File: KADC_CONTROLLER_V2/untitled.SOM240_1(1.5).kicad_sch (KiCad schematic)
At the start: 24 parts, among them J10 ADM6-60-01.5-L-4-2-A-TR, J7 1766453, SW2 SW_MEC_5G

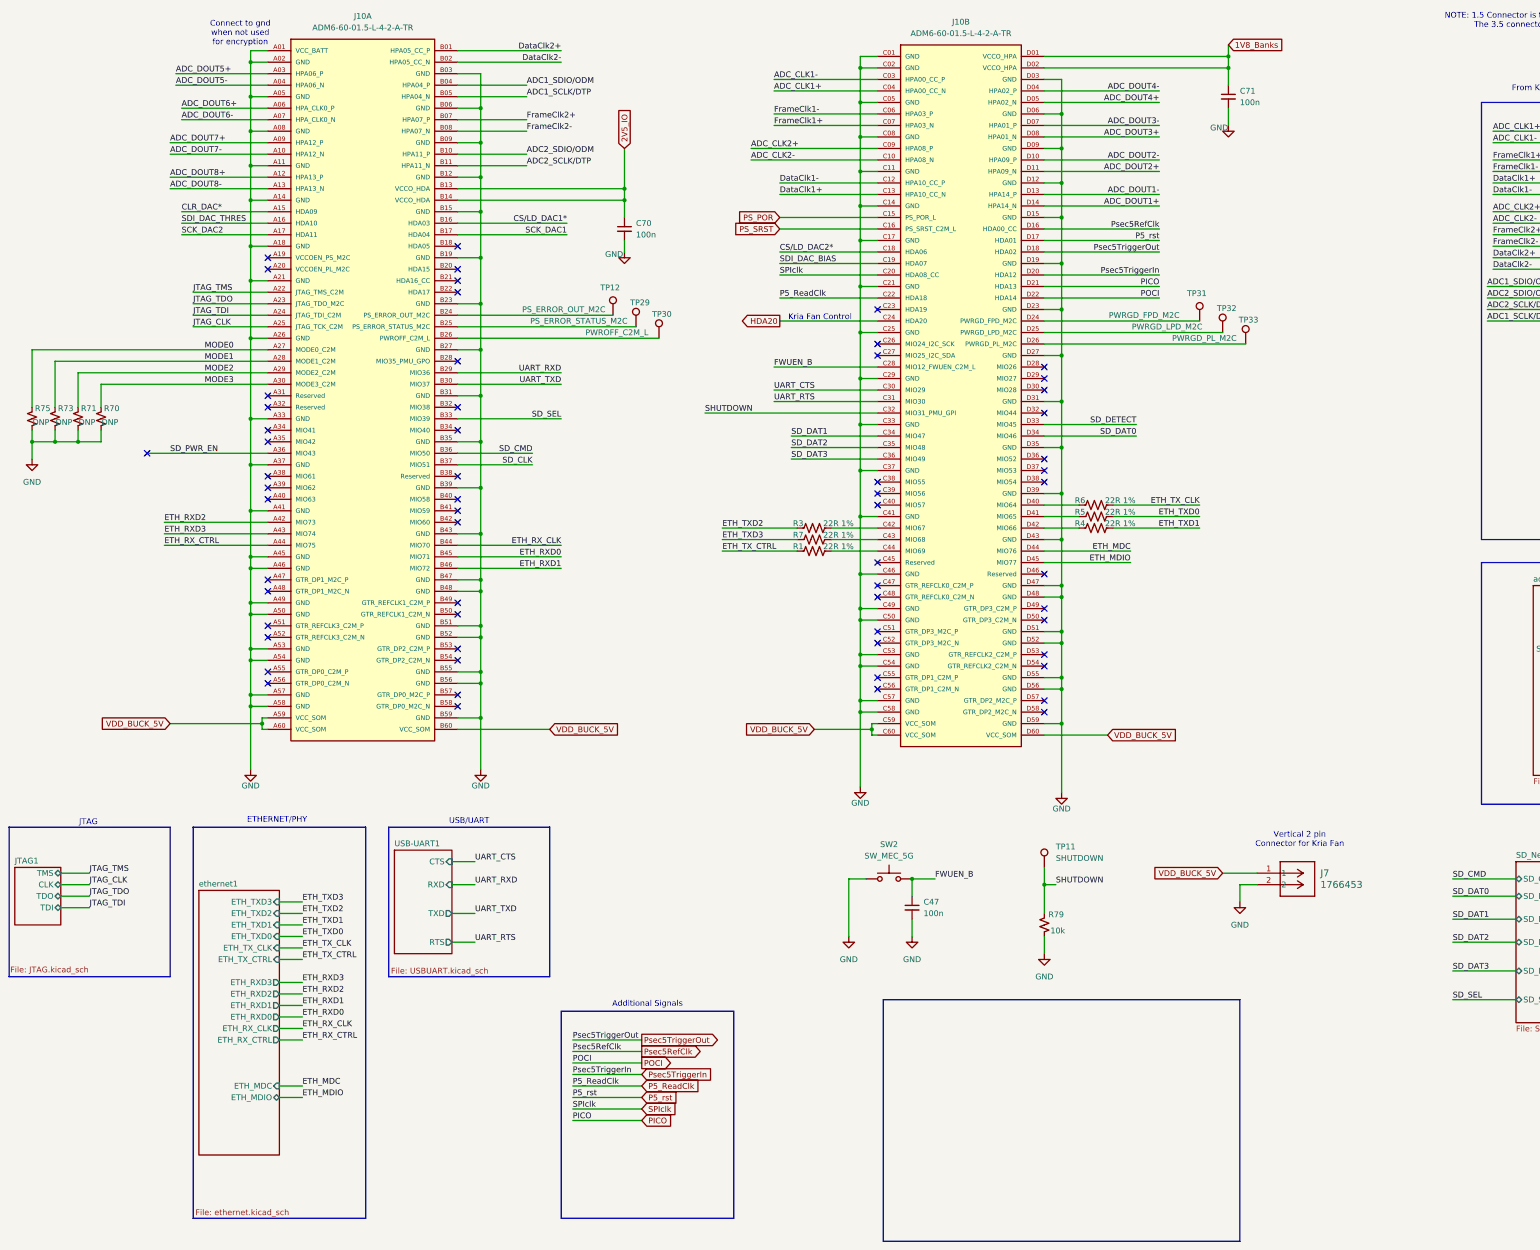
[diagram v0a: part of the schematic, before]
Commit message: many updates
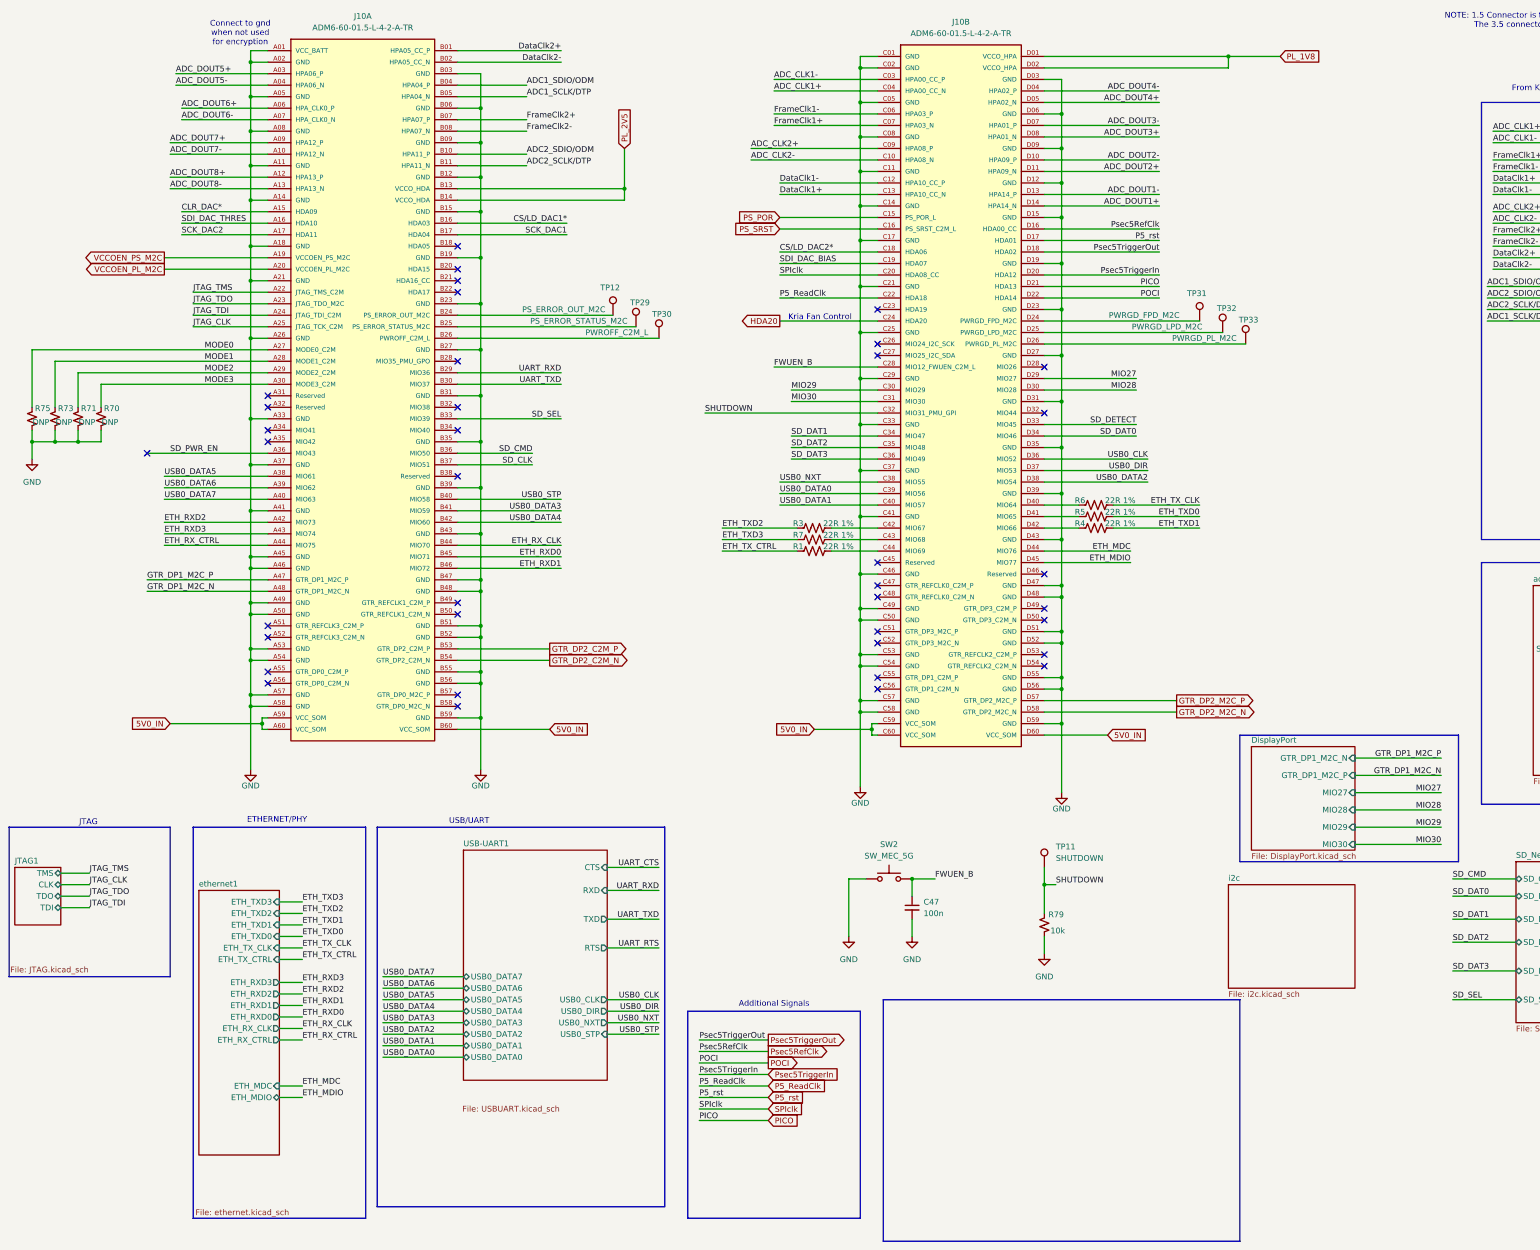
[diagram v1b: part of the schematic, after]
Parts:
- removed C70, C71: 100n, Capacitor_SMD:C_0603_1608Metric, symbol Device:C_Small
- removed J7: 1766453, 1766453:CONN_1766453, symbol PSEC5_ctrlbd:1766453
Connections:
- net UART_CTS: no longer J10.C30 (MIO29)
- net UART_RTS: no longer J10.C31 (MIO30)
- net VCCOEN_PS_M2C: now reaches J10.A19 (VCCOEN_PS_M2C)
- net VCCOEN_PL_M2C: now reaches J10.A20 (VCCOEN_PL_M2C)
- net USB0_DATA5: now reaches J10.A38 (MIO61)
- net USB0_DATA6: now reaches J10.A39 (MIO62)
- net USB0_DATA7: now reaches J10.A40 (MIO63)
- net GTR_DP1_M2C_P: now reaches J10.A47 (GTR_DP1_M2C_P)
- net GTR_DP1_M2C_N: now reaches J10.A48 (GTR_DP1_M2C_N)
- net USB0_STP: now reaches J10.B40 (MIO58)
- net USB0_DATA3: now reaches J10.B41 (MIO59)
- net USB0_DATA4: now reaches J10.B42 (MIO60)
- net GTR_DP2_C2M_P: now reaches J10.B53 (GTR_DP2_C2M_P)
- net GTR_DP2_C2M_N: now reaches J10.B54 (GTR_DP2_C2M_N)
- net USB0_NXT: now reaches J10.C38 (MIO55)
- net USB0_DATA0: now reaches J10.C39 (MIO56)
- net USB0_DATA1: now reaches J10.C40 (MIO57)
- net MIO27: now reaches J10.D29 (MIO27)
- net MIO28: now reaches J10.D30 (MIO28)
- net USB0_CLK: now reaches J10.D36 (MIO52)
- net USB0_DIR: now reaches J10.D37 (MIO53)
- net USB0_DATA2: now reaches J10.D38 (MIO54)
- net GTR_DP2_M2C_P: now reaches J10.D57 (GTR_DP2_M2C_P)
- net GTR_DP2_M2C_N: now reaches J10.D58 (GTR_DP2_M2C_N)
- net 1V8_Banks renamed PL_1V8
- net 2V5_IO renamed PL_2V5
- net VDD_BUCK_5V renamed 5V0_IN
- new net MIO29: J10.C30 (MIO29)
- new net MIO30: J10.C31 (MIO30)
- no-connect marks 60 -> 38
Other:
- added sheet DisplayPort (DisplayPort.kicad_sch)
- added sheet i2c (i2c.kicad_sch)
- sheet USB-UART1 ports: added USB0_CLK, USB0_DATA0, USB0_DATA1, USB0_DATA2, USB0_DATA3, USB0_DATA4, USB0_DATA5, USB0_DATA6, USB0_DATA7, USB0_DIR, USB0_NXT, USB0_STP; removed none
- note removed: "Vertical 2 pin Connector for Kria Fan"

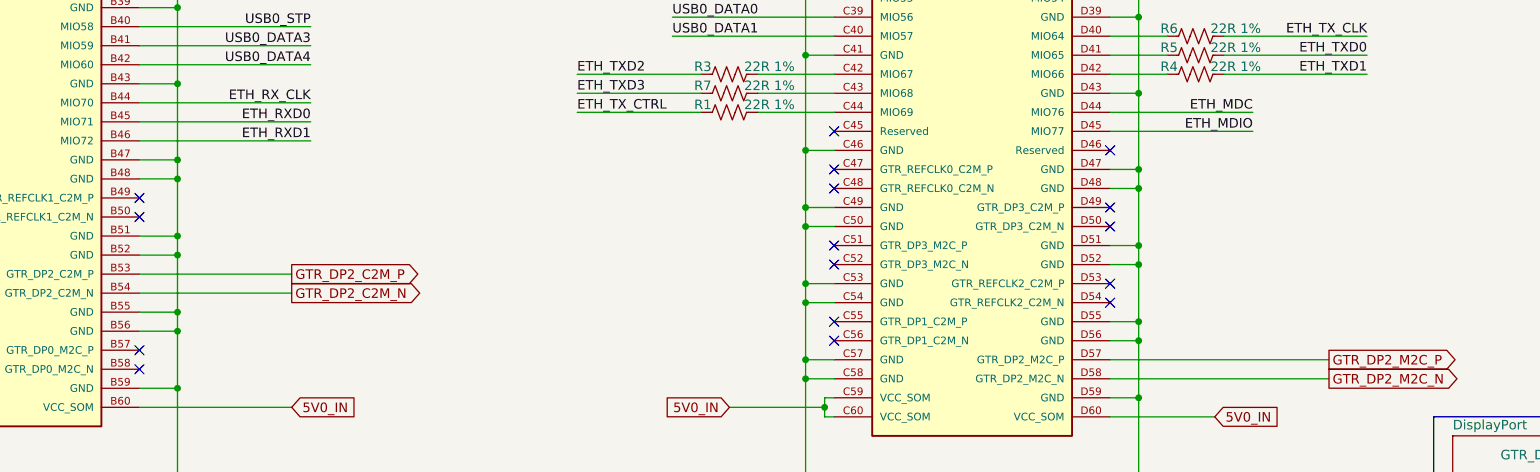
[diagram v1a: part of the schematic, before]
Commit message: More Things
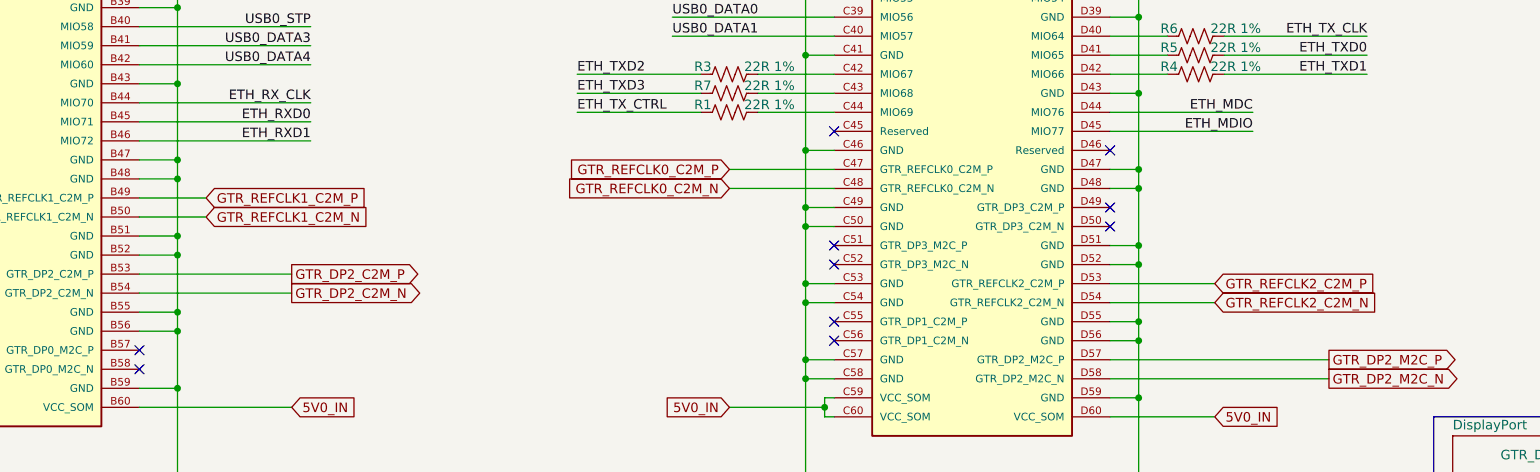
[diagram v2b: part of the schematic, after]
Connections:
- net GTR_REFCLK1_C2M_P: now reaches J10.B49 (GTR_REFCLK1_C2M_P)
- net GTR_REFCLK1_C2M_N: now reaches J10.B50 (GTR_REFCLK1_C2M_N)
- net GTR_REFCLK0_C2M_P: now reaches J10.C47 (GTR_REFCLK0_C2M_P)
- net GTR_REFCLK0_C2M_N: now reaches J10.C48 (GTR_REFCLK0_C2M_N)
- net GTR_REFCLK2_C2M_P: now reaches J10.D53 (GTR_REFCLK2_C2M_P)
- net GTR_REFCLK2_C2M_N: now reaches J10.D54 (GTR_REFCLK2_C2M_N)
- no-connect marks 38 -> 32
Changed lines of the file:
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@@
 	)
 	(no_connect
-		(at 121.92 146.05)
-	)
-	(no_connect
-		(at 214.63 142.24)
-	)
-	(no_connect
 		(at 121.92 72.39)
 	)
 	(no_connect
-		(at 121.92 143.51)
-	)
-	(no_connect
 		(at 121.92 100.33)
 	)
@@
 	)
 	(no_connect
-		(at 251.46 157.48)
-	)
-	(no_connect
 		(at 121.92 105.41)
 	)
@@
 	)
 	(no_connect
-		(at 251.46 154.94)
-	)
-	(no_connect
 		(at 121.92 90.17)
 	)
@@
 	)
 	(no_connect
-		(at 214.63 139.7)
-	)
-	(no_connect
 		(at 80.01 161.29)
 	)
@@
 	(wire
 		(pts
+			(xy 200.66 142.24) (xy 214.63 142.24)
+		)
+		(stroke
+			(width 0)
+			(type default)
+		)
+	)
+	(wire
+		(pts
+			(xy 121.92 146.05) (xy 130.81 146.05)
+		)
+		(stroke
+			(width 0)
+			(type default)
+		)
+	)
+	(wire
+		(pts
 			(xy 76.2 146.05) (xy 80.01 146.05)
 		)
@@
 	(wire
 		(pts
+			(xy 251.46 154.94) (xy 265.43 154.94)
+		)
+		(stroke
+			(width 0)
+			(type default)
+		)
+	)
+	(wire
+		(pts
 			(xy 121.92 21.59) (xy 144.78 21.59)
 		)
@@
 	(wire
 		(pts
+			(xy 121.92 143.51) (xy 130.81 143.51)
+		)
+		(stroke
+			(width 0)
+			(type default)
+		)
+	)
+	(wire
+		(pts
 			(xy 191.77 27.94) (xy 214.63 27.94)
 		)
@@
 	(wire
 		(pts
+			(xy 251.46 157.48) (xy 265.43 157.48)
+		)
+		(stroke
+			(width 0)
+			(type default)
+		)
+	)
+	(wire
+		(pts
 			(xy 76.2 135.89) (xy 76.2 143.51)
 		)
@@
 	(wire
 		(pts
+			(xy 200.66 139.7) (xy 214.63 139.7)
+		)
+		(stroke
+			(width 0)
+			(type default)
+		)
+	)
+	(wire
+		(pts
 			(xy 255.27 43.18) (xy 255.27 50.8)
 		)
@@
 		)
 	)
+	(global_label "GTR_REFCLK1_C2M_P"
+		(shape input)
+		(at 130.81 143.51 0)
+		(fields_autoplaced yes)
+		(effects
+			(font
+				(size 1.27 1.27)
+			)
+			(justify left)
+		)
+		(property "Intersheetrefs" "${INTERSHEET_REFS}"
+			(at 153.6917 143.51 0)
+			(hide yes)
+			(show_name no)
+			(do_not_autoplace no)
+			(effects
+				(font
+					(size 1.27 1.27)
+				)
+				(justify left)
+			)
+		)
+	)
 	(global_label "GTR_DP2_C2M_P"
 		(shape output)
@@
 		)
 	)
+	(global_label "GTR_REFCLK1_C2M_N"
+		(shape input)
+		(at 130.81 146.05 0)
+		(fields_autoplaced yes)
+		(effects
+			(font
+				(size 1.27 1.27)
+			)
+			(justify left)
+		)
+		(property "Intersheetrefs" "${INTERSHEET_REFS}"
+			(at 153.7522 146.05 0)
+			(hide yes)
+			(show_name no)
+			(do_not_autoplace no)
+			(effects
+				(font
+					(size 1.27 1.27)
+				)
+				(justify left)
+			)
+		)
+	)
 	(global_label "SPIclk"
 		(shape input)
@@
 		)
 	)
+	(global_label "GTR_REFCLK0_C2M_N"
+		(shape input)
+		(at 200.66 142.24 180)
+		(fields_autoplaced yes)
+		(effects
+			(font
+				(size 1.27 1.27)
+			)
+			(justify right)
+		)
+		(property "Intersheetrefs" "${INTERSHEET_REFS}"
+			(at 177.7178 142.24 0)
+			(hide yes)
+			(show_name no)
+			(do_not_autoplace no)
+			(effects
+				(font
+					(size 1.27 1.27)
+				)
+				(justify right)
+			)
+		)
+	)
+	(global_label "GTR_REFCLK0_C2M_P"
+		(shape input)
+		(at 200.66 139.7 180)
+		(fields_autoplaced yes)
+		(effects
+			(font
+				(size 1.27 1.27)
+			)
+			(justify right)
+		)
+		(property "Intersheetrefs" "${INTERSHEET_REFS}"
+			(at 177.7783 139.7 0)
+			(hide yes)
+			(show_name no)
+			(do_not_autoplace no)
+			(effects
+				(font
+					(size 1.27 1.27)
+				)
+				(justify right)
+			)
+		)
+	)
+	(global_label "GTR_REFCLK2_C2M_N"
+		(shape input)
+		(at 265.43 157.48 0)
+		(fields_autoplaced yes)
+		(effects
+			(font
+				(size 1.27 1.27)
+			)
+			(justify left)
+		)
+		(property "Intersheetrefs" "${INTERSHEET_REFS}"
+			(at 288.3722 157.48 0)
+			(hide yes)
+			(show_name no)
+			(do_not_autoplace no)
+			(effects
+				(font
+					(size 1.27 1.27)
+				)
+				(justify left)
+			)
+		)
+	)
 	(global_label "5V0_IN"
 		(shape input)
@@
 			)
 		)
+	)
+	(global_label "GTR_REFCLK2_C2M_P"
+		(shape input)
+		(at 265.43 154.94 0)
+		(fields_autoplaced yes)
+		(effects
+			(font
+				(size 1.27 1.27)
+			)
+			(justify left)
+		)
+		(property "Intersheetrefs" "${INTERSHEET_REFS}"
+			(at 288.3117 154.94 0)
+			(hide yes)
+			(show_name no)
+			(do_not_autoplace no)
+			(effects
+				(font
+					(size 1.27 1.27)
+				)
+				(justify left)
+			)
+		)
